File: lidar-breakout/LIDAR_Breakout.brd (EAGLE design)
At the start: 36.5 x 88 mm, 82 parts

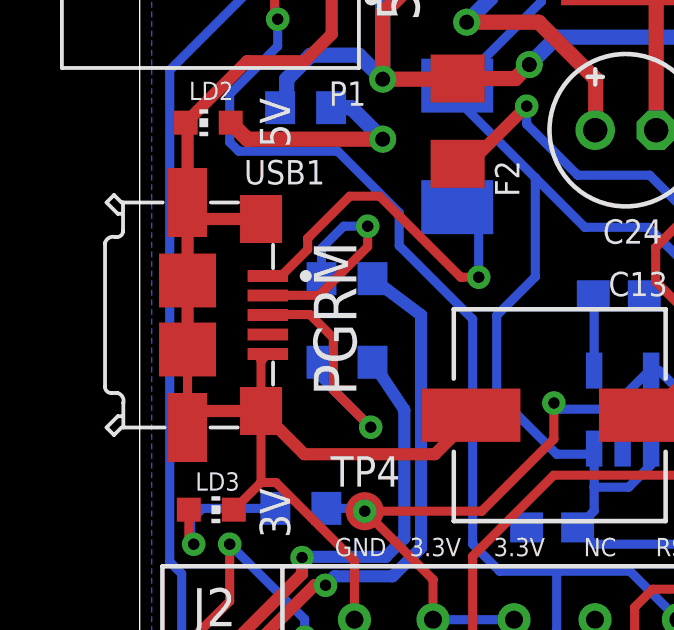
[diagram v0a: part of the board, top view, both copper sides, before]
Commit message: Reran cam
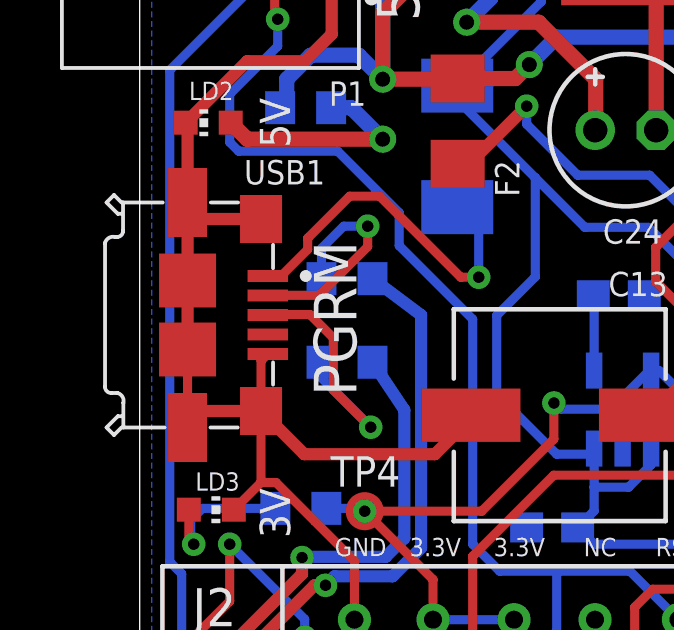
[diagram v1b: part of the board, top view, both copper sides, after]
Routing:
- net GND: track 249.3 -> 247.2 mm
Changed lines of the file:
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@@
 <contactref element="USB1" pad="10"/>
 <wire x1="1.595" y1="42.19" x2="1.595" y2="39.89" width="0.4064" layer="1"/>
-<wire x1="1.595" y1="43.9" x2="1.595" y2="42.19" width="0.4064" layer="1"/>
-<wire x1="4.045" y1="44.24" x2="2.4" y2="44.24" width="0.4064" layer="1"/>
-<wire x1="2.4" y1="44.24" x2="1.555" y2="44.24" width="0.4064" layer="1"/>
-<wire x1="4.045" y1="37.84" x2="1.935" y2="37.84" width="0.4064" layer="1"/>
 <wire x1="5.485" y1="36.4" x2="4.045" y2="37.84" width="0.4064" layer="1"/>
 <wire x1="9.8409" y1="36.4" x2="5.485" y2="36.4" width="0.4064" layer="1"/>
@@
 <wire x1="6.4" y1="50.4" x2="6.4" y2="52.527" width="0.4064" layer="1"/>
 <wire x1="6.4" y1="52.527" x2="6.327" y2="52.6" width="0.4064" layer="1"/>
-<wire x1="1.595" y1="44.79" x2="2.145" y2="44.24" width="0.3048" layer="1"/>
-<wire x1="2.145" y1="44.24" x2="2.4" y2="44.24" width="0.3048" layer="1"/>
 <wire x1="1.595" y1="39.89" x2="1.595" y2="37.29" width="0.3048" layer="1"/>
-<wire x1="1.595" y1="37.29" x2="2.145" y2="37.84" width="0.3048" layer="1"/>
-<wire x1="2.145" y1="37.84" x2="4.045" y2="37.84" width="0.3048" layer="1"/>
 <wire x1="3.128" y1="61.169" x2="4" y2="62.041" width="0.3048" layer="1"/>
 <wire x1="4" y1="62.041" x2="4" y2="64.7" width="0.3048" layer="1"/>
 <wire x1="4.54396875" y1="35.45603125" x2="4.045" y2="35.45603125" width="0.3048" layer="1"/>
 <wire x1="7.15831875" y1="32.84168125" x2="4.54396875" y2="35.45603125" width="0.3048" layer="1"/>
+<wire x1="4.045" y1="44.24" x2="2.145" y2="44.24" width="0.4064" layer="1"/>
+<wire x1="2.145" y1="44.24" x2="1.595" y2="44.79" width="0.4064" layer="1"/>
+<wire x1="1.595" y1="44.79" x2="1.595" y2="42.19" width="0.4064" layer="1"/>
+<wire x1="1.595" y1="37.29" x2="2.145" y2="37.84" width="0.4064" layer="1"/>
+<wire x1="2.145" y1="37.84" x2="4.045" y2="37.84" width="0.4064" layer="1"/>
 </signal>
 <signal name="RST_MC">
